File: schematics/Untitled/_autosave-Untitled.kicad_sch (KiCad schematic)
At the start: 34 parts, among them M1 Motor_DC, Q1 NPN, Q2 PNP, Q3 NPN, Q4 NPN, Q5 NPN, Q6 NPN, U1 INA260, U2 XL1509-3.3, U3 ESP32-WROOM-32

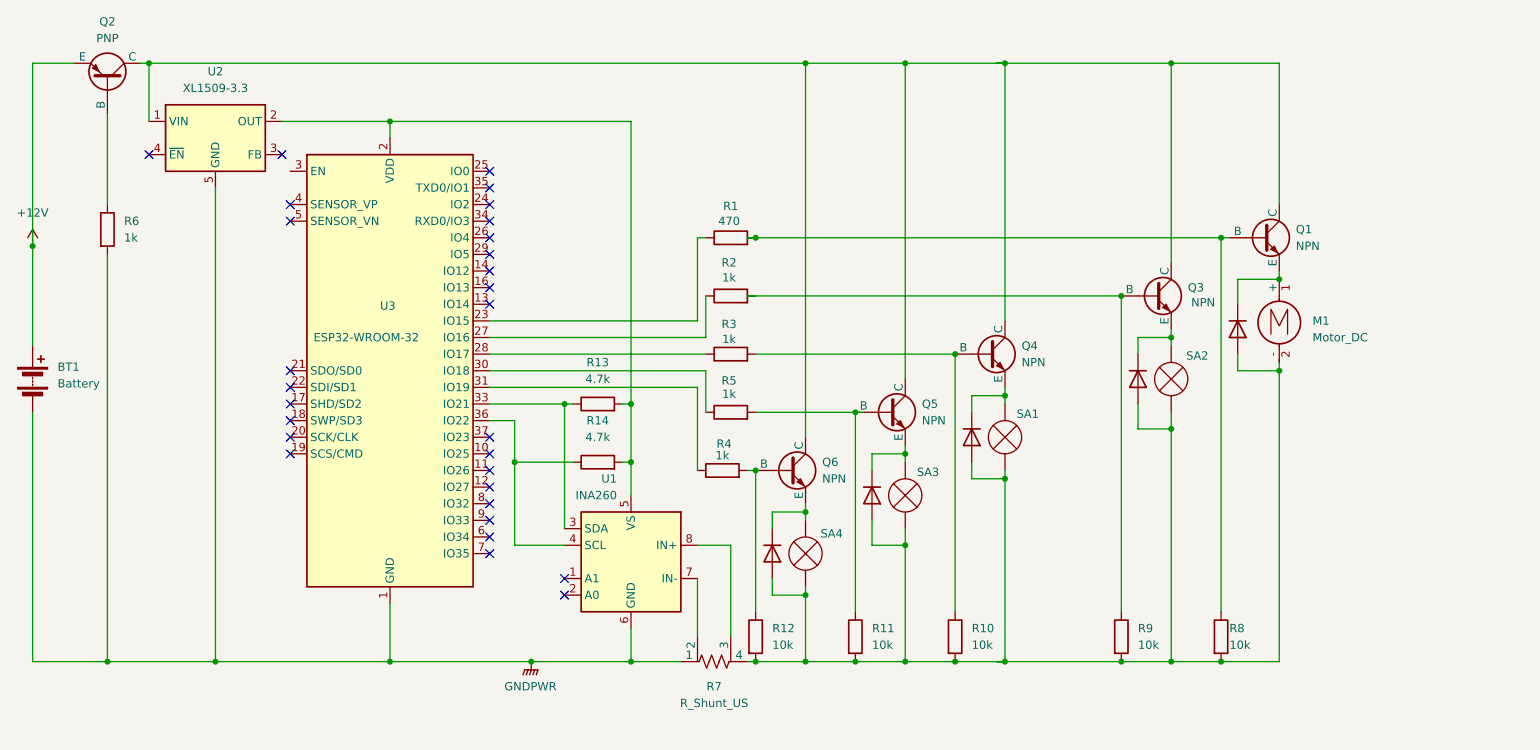
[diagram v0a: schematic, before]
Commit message: Updates
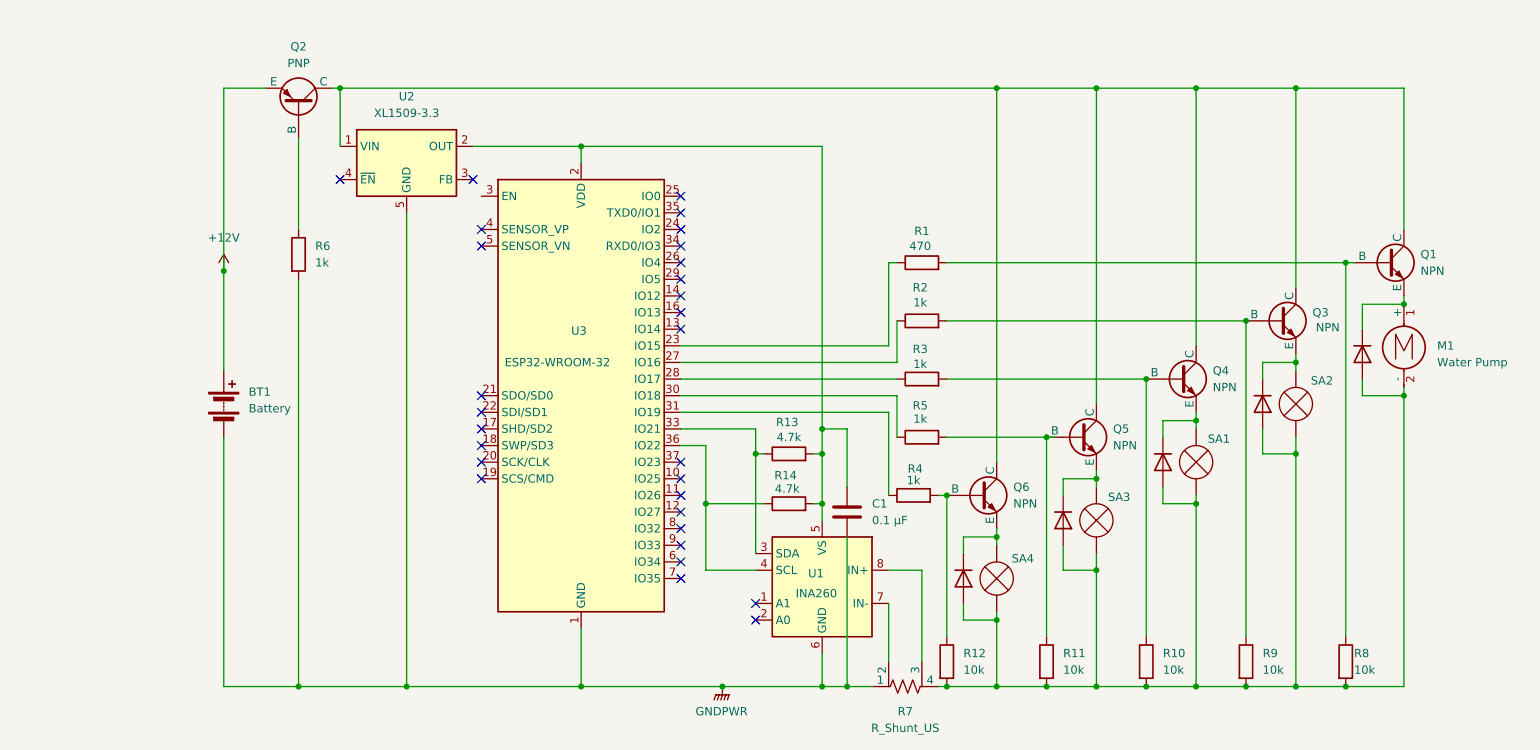
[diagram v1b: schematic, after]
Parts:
- added C1: 0.1 µF, symbol Device:C
- M1: value Motor_DC -> Water Pump
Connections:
- net GNDPWR: now also C1.2
- net at R13.2, R14.2, U1.5 (VS)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: now also C1.1
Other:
- moved on the sheet: BT1, M1, Q1, Q2, Q3, Q4, Q5, Q6, R1, R10, R11, R12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
